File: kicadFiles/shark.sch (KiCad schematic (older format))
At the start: 267 parts, among them J1 TYPE-C-31-M12_13, J2 Conn_01x04_Male, J3 Conn_01x04_Male, J4 Conn_01x04_Male, J5 Conn_01x06_Male, Q1 AO4406AL, SW1 MXSwitch, SW10 MXSwitch, SW11 MXSwitch, SW12 MXSwitch, SW13 MXSwitch, SW14 MXSwitch, SW15 MXSwitch, SW16 MXSwitch, SW17 MXSwitch, SW18 MXSwitch, SW19 MXSwitch, SW2 MXSwitch, SW20 MXSwitch, SW21 MXSwitch, SW22 MXSwitch, SW23 MXSwitch, SW24 MXSwitch, SW25 MXSwitch, SW26 MXSwitch, SW27 MXSwitch, SW28 MXSwitch, SW29 MXSwitch, SW3 MXSwitch, SW30 MXSwitch, SW31 MXSwitch, SW32 MXSwitch, SW33 MXSwitch, SW34 MXSwitch, SW35 MXSwitch, SW36 MXSwitch, SW37 MXSwitch, SW38 MXSwitch, SW39 MXSwitch, SW4 MXSwitch, SW40 MXSwitch, SW41 MXSwitch, SW42 MXSwitch, SW43 MXSwitch, SW44 MXSwitch, SW45 MXSwitch, SW46 MXSwitch, SW47 MXSwitch, SW48 MXSwitch, SW49 MXSwitch, SW5 MXSwitch, SW50 MXSwitch, SW51 MXSwitch, SW6 MXSwitch, SW7 MXSwitch, SW8 MXSwitch, SW9 MXSwitch, U1 STM32F303-LQFP48, U2 MCP1700-3302E_SOT23, U3 USBLC6-2SC6, Y1 8MHz

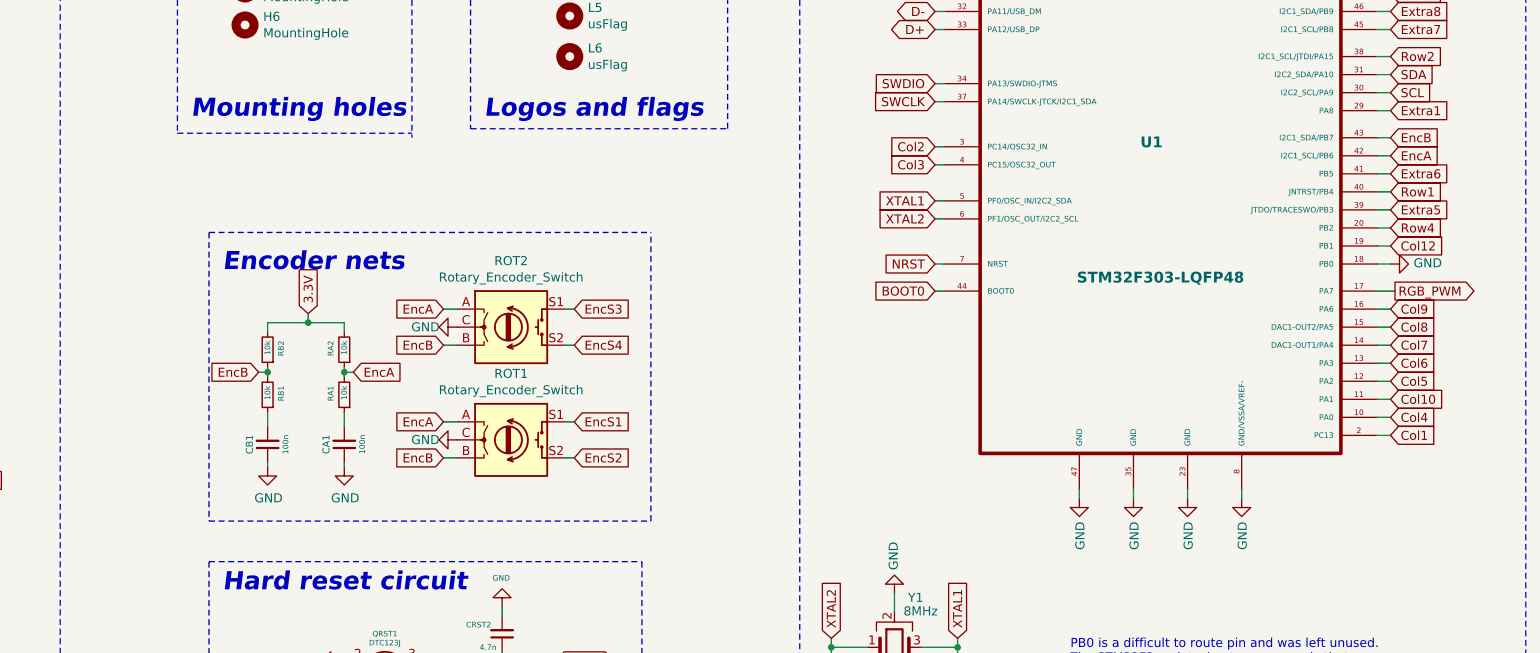
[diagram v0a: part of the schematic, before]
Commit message: [Update] Renamed some nets and re-routed some traces related to the encoders for better understanding of the circuit and noice cancelling
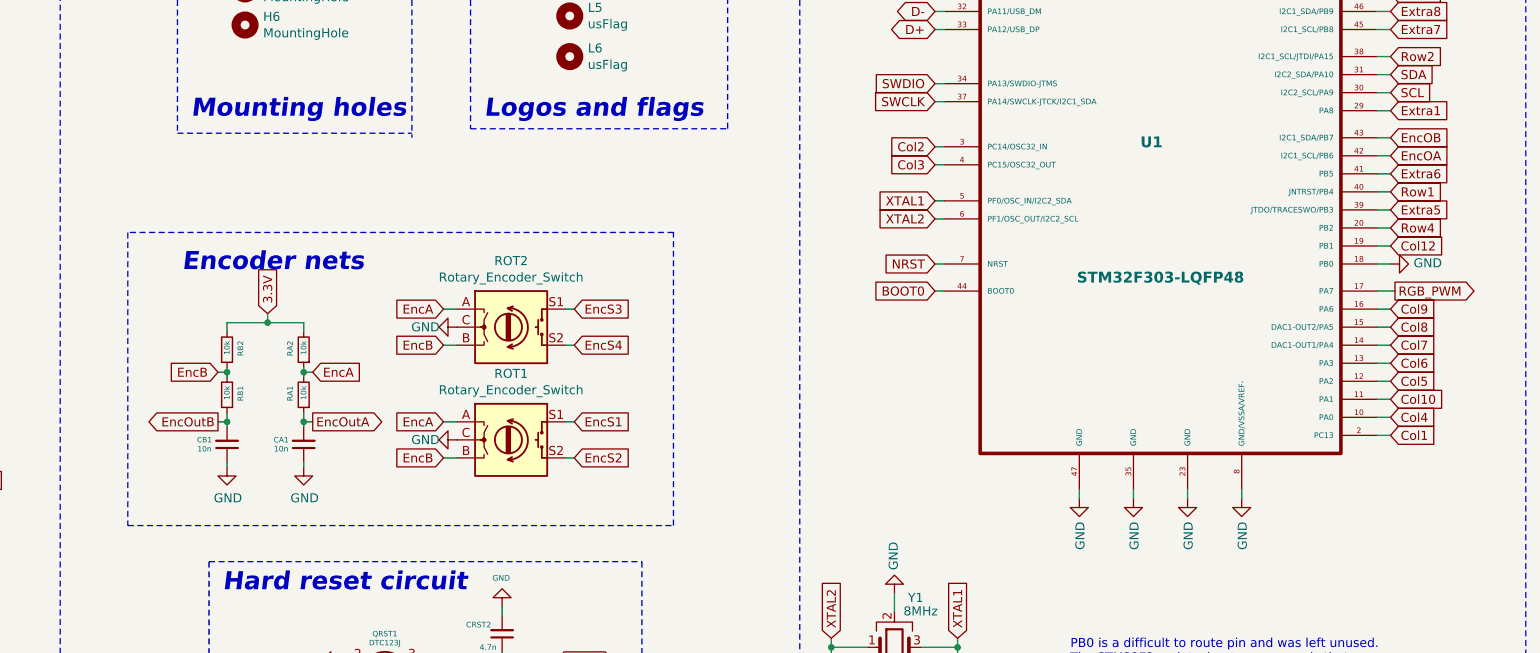
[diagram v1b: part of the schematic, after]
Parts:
- CA1, CB1: value 100n -> 10n
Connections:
- net EncA: no longer U1.42 (I2C1_SCL/PB6)
- net EncB: no longer U1.43 (I2C1_SDA/PB7)
- net EncOutB: now reaches CB1.2, RB1.1
- net EncOutA: now reaches CA1.2, RA1.1
- new net EncOA: U1.42 (I2C1_SCL/PB6)
- new net EncOB: U1.43 (I2C1_SDA/PB7)
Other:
- moved on the sheet: CA1, CB1, RA1, RA2, RB1, RB2
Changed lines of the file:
@@
 L Device:C_Small CB1
 U 1 1 5CF05817
-P 15350 6475
-F 0 "CB1" V 15450 6475 39  0000 C CNN
-F 1 "100n" V 15250 6475 31  0000 C CNN
-F 2 "Capacitor_SMD:C_0805_2012Metric_Pad1.15x1.40mm_HandSolder" H 15350 6475 50  0001 C CNN
-F 3 "~" H 15350 6475 50  0001 C CNN
-	1    15350 6475
+P 15125 6475
+F 0 "CB1" H 15250 6450 30  0000 C CNN
+F 1 "10n" H 15250 6500 30  0000 C CNN
+F 2 "Capacitor_SMD:C_0805_2012Metric_Pad1.15x1.40mm_HandSolder" H 15125 6475 50  0001 C CNN
+F 3 "~" H 15125 6475 50  0001 C CNN
+	1    15125 6475
 	-1   0    0    1
 $EndComp
@@
 L Device:C_Small CA1
 U 1 1 5CF063CC
-P 15775 6475
-F 0 "CA1" V 15875 6475 39  0000 C CNN
-F 1 "100n" V 15675 6475 31  0000 C CNN
-F 2 "Capacitor_SMD:C_0805_2012Metric_Pad1.15x1.40mm_HandSolder" H 15775 6475 50  0001 C CNN
-F 3 "~" H 15775 6475 50  0001 C CNN
-	1    15775 6475
+P 15550 6475
+F 0 "CA1" H 15675 6450 30  0000 C CNN
+F 1 "10n" H 15675 6500 31  0000 C CNN
+F 2 "Capacitor_SMD:C_0805_2012Metric_Pad1.15x1.40mm_HandSolder" H 15550 6475 50  0001 C CNN
+F 3 "~" H 15550 6475 50  0001 C CNN
+	1    15550 6475
 	-1   0    0    1
 $EndComp
@@
 L power:GND #PWR06
 U 1 1 5CF06B2F
-P 15350 6600
-F 0 "#PWR06" H 15350 6350 50  0001 C CNN
-F 1 "GND" H 15355 6427 50  0000 C CNN
-F 2 "" H 15350 6600 50  0001 C CNN
-F 3 "" H 15350 6600 50  0001 C CNN
-	1    15350 6600
+P 15125 6600
+F 0 "#PWR06" H 15125 6350 50  0001 C CNN
+F 1 "GND" H 15130 6427 50  0000 C CNN
+F 2 "" H 15125 6600 50  0001 C CNN
+F 3 "" H 15125 6600 50  0001 C CNN
+	1    15125 6600
 	1    0    0    -1
 $EndComp
@@
 L power:GND #PWR07
 U 1 1 5CF07233
-P 15775 6600
-F 0 "#PWR07" H 15775 6350 50  0001 C CNN
-F 1 "GND" H 15780 6427 50  0000 C CNN
-F 2 "" H 15775 6600 50  0001 C CNN
-F 3 "" H 15775 6600 50  0001 C CNN
-	1    15775 6600
+P 15550 6600
+F 0 "#PWR07" H 15550 6350 50  0001 C CNN
+F 1 "GND" H 15555 6427 50  0000 C CNN
+F 2 "" H 15550 6600 50  0001 C CNN
+F 3 "" H 15550 6600 50  0001 C CNN
+	1    15550 6600
 	1    0    0    -1
 $EndComp
@@
 L Device:R_Small RA1
 U 1 1 5CF07838
-P 15775 6200
-F 0 "RA1" V 15850 6150 31  0000 L CNN
-F 1 "10k" V 15775 6150 31  0000 L CNN
-F 2 "acheronComponents:R_1026" H 15775 6200 50  0001 C CNN
-F 3 "~" H 15775 6200 50  0001 C CNN
-	1    15775 6200
-	-1   0    0    1
-$EndComp
-$Comp
-L Device:R_Small RB1
-U 1 1 5CFD7290
-P 15350 6200
-F 0 "RB1" V 15275 6150 31  0000 L CNN
-F 1 "10k" V 15350 6150 31  0000 L CNN
-F 2 "acheronComponents:R_1026" H 15350 6200 50  0001 C CNN
-F 3 "~" H 15350 6200 50  0001 C CNN
-	1    15350 6200
-	-1   0    0    1
-$EndComp
-Wire Wire Line
-	15350 6375 15350 6300
-Wire Wire Line
-	15775 6300 15775 6375
-Wire Wire Line
-	15775 6575 15775 6600
-Wire Wire Line
-	15350 6575 15350 6600
+P 15550 6200
+F 0 "RA1" V 15625 6150 31  0000 L CNN
+F 1 "10k" V 15550 6150 31  0000 L CNN
+F 2 "acheronComponents:R_1026" H 15550 6200 50  0001 C CNN
+F 3 "~" H 15550 6200 50  0001 C CNN
+	1    15550 6200
+	-1   0    0    1
+$EndComp
+Wire Wire Line
+	15125 6375 15125 6350
+Wire Wire Line
+	15550 6300 15550 6350
+Wire Wire Line
+	15550 6575 15550 6600
+Wire Wire Line
+	15125 6575 15125 6600
 $Comp
 L Device:R_Small RB2
 U 1 1 5D1DE77E
-P 15350 5950
-F 0 "RB2" V 15275 5900 31  0000 L CNN
-F 1 "10k" V 15350 5900 31  0000 L CNN
-F 2 "acheronComponents:R_1026" H 15350 5950 50  0001 C CNN
-F 3 "~" H 15350 5950 50  0001 C CNN
-	1    15350 5950
+P 15125 5950
+F 0 "RB2" V 15050 5900 31  0000 L CNN
+F 1 "10k" V 15125 5900 31  0000 L CNN
+F 2 "acheronComponents:R_1026" H 15125 5950 50  0001 C CNN
+F 3 "~" H 15125 5950 50  0001 C CNN
+	1    15125 5950
 	-1   0    0    1
 $EndComp
@@
 L Device:R_Small RA2
 U 1 1 5D1DF5E6
-P 15775 5950
-F 0 "RA2" V 15850 5900 31  0000 L CNN
-F 1 "10k" V 15775 5900 31  0000 L CNN
-F 2 "acheronComponents:R_1026" H 15775 5950 50  0001 C CNN
-F 3 "~" H 15775 5950 50  0001 C CNN
-	1    15775 5950
-	-1   0    0    1
-$EndComp
-Wire Wire Line
-	15350 6050 15350 6075
-Wire Wire Line
-	15775 6050 15775 6075
-Wire Wire Line
-	15350 5850 15350 5800
-Wire Wire Line
-	15350 5800 15575 5800
-Wire Wire Line
-	15775 5800 15775 5850
-Wire Wire Line
-	15575 5800 15575 5750
-Connection ~ 15575 5800
-Wire Wire Line
-	15575 5800 15775 5800
-Text GLabel 15300 6075 0    50   Input ~ 0
-EncB
-Text GLabel 15825 6075 2    50   Input ~ 0
-EncA
-Text GLabel 15575 5750 1    50   Input ~ 0
+P 15550 5950
+F 0 "RA2" V 15625 5900 31  0000 L CNN
+F 1 "10k" V 15550 5900 31  0000 L CNN
+F 2 "acheronComponents:R_1026" H 15550 5950 50  0001 C CNN
+F 3 "~" H 15550 5950 50  0001 C CNN
+	1    15550 5950
+	-1   0    0    1
+$EndComp
+Wire Wire Line
+	15125 6050 15125 6075
+Wire Wire Line
+	15550 6050 15550 6075
+Wire Wire Line
+	15125 5850 15125 5800
+Wire Wire Line
+	15125 5800 15350 5800
+Wire Wire Line
+	15550 5800 15550 5850
+Wire Wire Line
+	15350 5800 15350 5750
+Connection ~ 15350 5800
+Wire Wire Line
+	15350 5800 15550 5800
+Text GLabel 15350 5750 1    50   Input ~ 0
 3.3V
 Wire Wire Line
-	15300 6075 15350 6075
-Connection ~ 15350 6075
-Wire Wire Line
-	15350 6075 15350 6100
-Wire Wire Line
-	15825 6075 15775 6075
-Connection ~ 15775 6075
-Wire Wire Line
-	15775 6075 15775 6100
-Wire Notes Line width 20
-	17475 6900 17475 5300
-Text Notes 15100 5525 0    100  Italic 20
+	15075 6075 15125 6075
+Connection ~ 15125 6075
+Wire Wire Line
+	15125 6075 15125 6100
+Wire Wire Line
+	15600 6075 15550 6075
+Connection ~ 15550 6075
+Wire Wire Line
+	15550 6075 15550 6100
+Text Notes 14875 5525 0    100  Italic 20
 Encoder nets
 Connection ~ 2475 3275
@@
 	1900 7050 1975 7050
 Connection ~ 1975 7050
-Wire Notes Line width 20
-	15025 5300 17475 5300
-Wire Notes Line width 20
-	15025 5300 15025 6900
-Wire Notes Line width 20
-	15025 6900 17475 6900
 Wire Wire Line
 	16325 6550 16400 6550
@@
 	21575 4775 21500 4775
 Text GLabel 21575 4775 2    50   Input ~ 0
-EncB
+EncOB
 Text GLabel 21575 4875 2    50   Input ~ 0
-EncA
+EncOA
 Wire Wire Line
 	21600 5625 21500 5625
@@
 	19850 6725 19850 6775
 $Comp
-L power:GND #PWR?
+L power:GND #PWR0115
 U 1 1 5D4FC297
 P 21575 5475
-F 0 "#PWR?" H 21575 5225 50  0001 C CNN
+F 0 "#PWR0115" H 21575 5225 50  0001 C CNN
 F 1 "GND" V 21580 5347 50  0000 R CNN
 F 2 "" H 21575 5475 50  0001 C CNN
@@
 Text Notes 19800 7775 0    50   ~ 0
 PB0 is a difficult to route pin and was left unused.\nThe STM32F3xx datasheet recommends that\nunused pins are grounded
+Text GLabel 15075 6075 0    50   Input ~ 0
+EncB
+Text GLabel 15600 6075 2    50   Input ~ 0
+EncA
+Text GLabel 15075 6350 0    50   Output ~ 0
+EncOutB
+Text GLabel 15600 6350 2    50   Output ~ 0
+EncOutA
+Wire Wire Line
+	15075 6350 15125 6350
+Connection ~ 15125 6350
+Wire Wire Line
+	15125 6350 15125 6300
+Wire Wire Line
+	15600 6350 15550 6350
+Connection ~ 15550 6350
+Wire Wire Line
+	15550 6350 15550 6375
+Wire Notes Line width 20
+	14575 5300 14575 6925
+Wire Notes Line width 20
+	14575 6925 17600 6925
+Wire Notes Line width 20
+	17600 6925 17600 5300
+Wire Notes Line width 20
+	17600 5300 14575 5300
+$Comp
+L Device:R_Small RB1
+U 1 1 5CFD7290
+P 15125 6200
+F 0 "RB1" V 15050 6150 31  0000 L CNN
+F 1 "10k" V 15125 6150 31  0000 L CNN
+F 2 "acheronComponents:R_1026" H 15125 6200 50  0001 C CNN
+F 3 "~" H 15125 6200 50  0001 C CNN
+	1    15125 6200
+	-1   0    0    1
+$EndComp
 $EndSCHEMATC

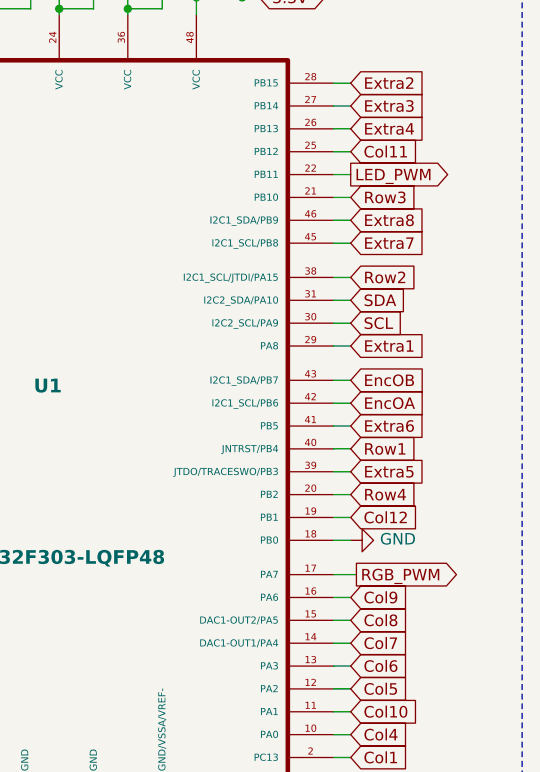
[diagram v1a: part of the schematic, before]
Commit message: Change pins in footprint
- The LED_PWM pin was changed to pin B7, which has PWM capability;
- The RGB_LED pin was changed to B6, which has SPI capability;
- Some col and row pins were change to accomodate those chamges;
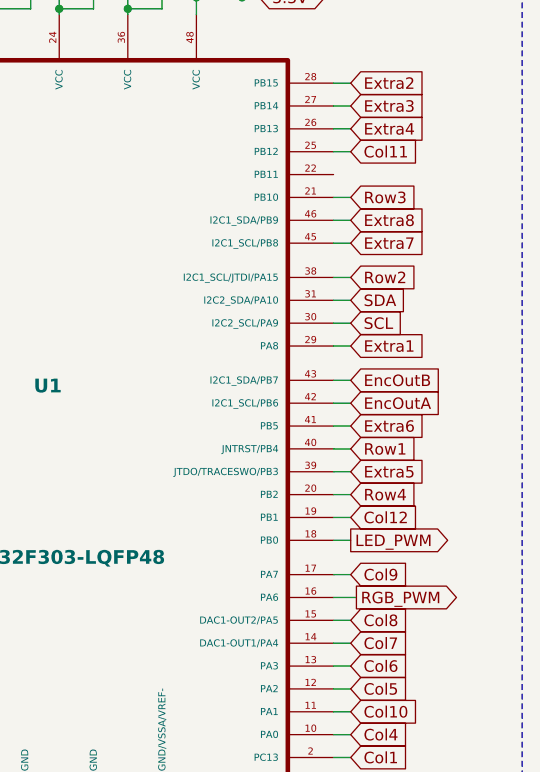
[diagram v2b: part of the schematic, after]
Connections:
- net EncOA is gone; now on net EncOutA: U1.42 (I2C1_SCL/PB6)
- net EncOB is gone; now on net EncOutB: U1.43 (I2C1_SDA/PB7)
- net Col9: now also U1.17 (PA7); no longer U1.16 (PA6)
- net GND: no longer U1.18 (PB0)
- net LED_PWM: now also U1.18 (PB0); no longer U1.22 (PB11)
- net RGB_PWM: now also U1.16 (PA6); no longer U1.17 (PA7)
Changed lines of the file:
@@
 EESchema Schematic File Version 4
 LIBS:shark-cache
-EELAYER 29 0
+EELAYER 30 0
 EELAYER END
 $Descr A2 23386 16535
@@
 	21575 4775 21500 4775
 Text GLabel 21575 4775 2    50   Input ~ 0
-EncOB
+EncOutB
 Text GLabel 21575 4875 2    50   Input ~ 0
-EncOA
+EncOutA
 Wire Wire Line
-	21600 5625 21500 5625
+	21600 5725 21500 5725
 Wire Wire Line
 	21575 5075 21500 5075
@@
 Row1
 Wire Wire Line
-	21575 5725 21500 5725
-Text GLabel 21575 5725 2    50   Input ~ 0
+	21575 5625 21500 5625
+Text GLabel 21575 5625 2    50   Input ~ 0
 Col9
 Wire Wire Line
@@
 Text GLabel 21575 6425 2    50   Input ~ 0
 Col1
-Text GLabel 21600 5625 2    50   Output ~ 0
+Text GLabel 21600 5725 2    50   Output ~ 0
 RGB_PWM
 Wire Wire Line
-	21575 3875 21500 3875
-Text GLabel 21575 3875 2    50   Output ~ 0
+	21575 5475 21500 5475
+Text GLabel 21575 5475 2    50   Output ~ 0
 LED_PWM
 Wire Wire Line
@@
 Wire Wire Line
 	19850 6725 19850 6775
-$Comp
-L power:GND #PWR0115
-U 1 1 5D4FC297
-P 21575 5475
-F 0 "#PWR0115" H 21575 5225 50  0001 C CNN
-F 1 "GND" V 21580 5347 50  0000 R CNN
-F 2 "" H 21575 5475 50  0001 C CNN
-F 3 "" H 21575 5475 50  0001 C CNN
-	1    21575 5475
-	0    -1   -1   0
-$EndComp
-Wire Wire Line
-	21575 5475 21500 5475
 Text Notes 19800 7775 0    50   ~ 0
 PB0 is a difficult to route pin and was left unused.\nThe STM32F3xx datasheet recommends that\nunused pins are grounded
